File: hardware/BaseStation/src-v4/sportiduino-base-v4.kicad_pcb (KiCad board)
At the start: 2 copper layers, 73 x 45 mm, 46 parts, among them SW1 SW_Reed, X1 Battery, X2 Prog, X3 RC522, X4 MINI RC522, X5 Charge

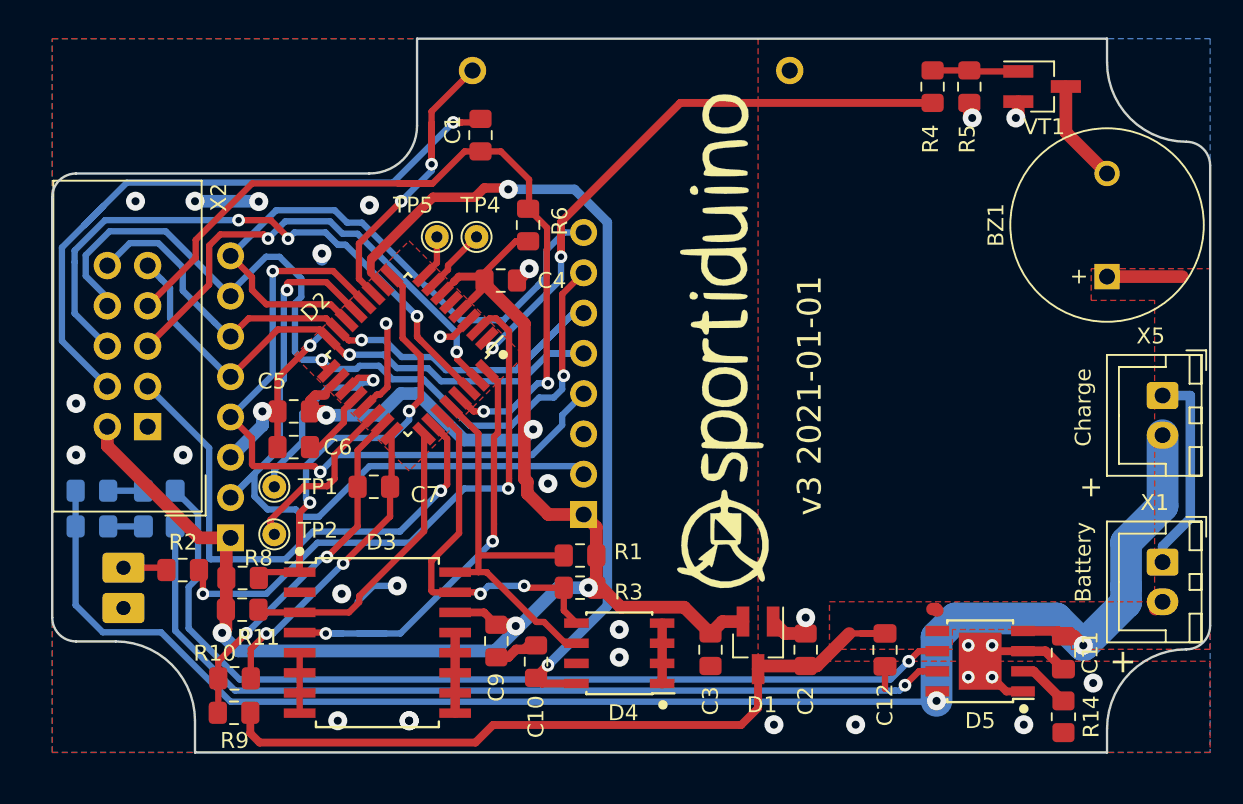
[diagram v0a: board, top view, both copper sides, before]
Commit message: New PCB (wip)
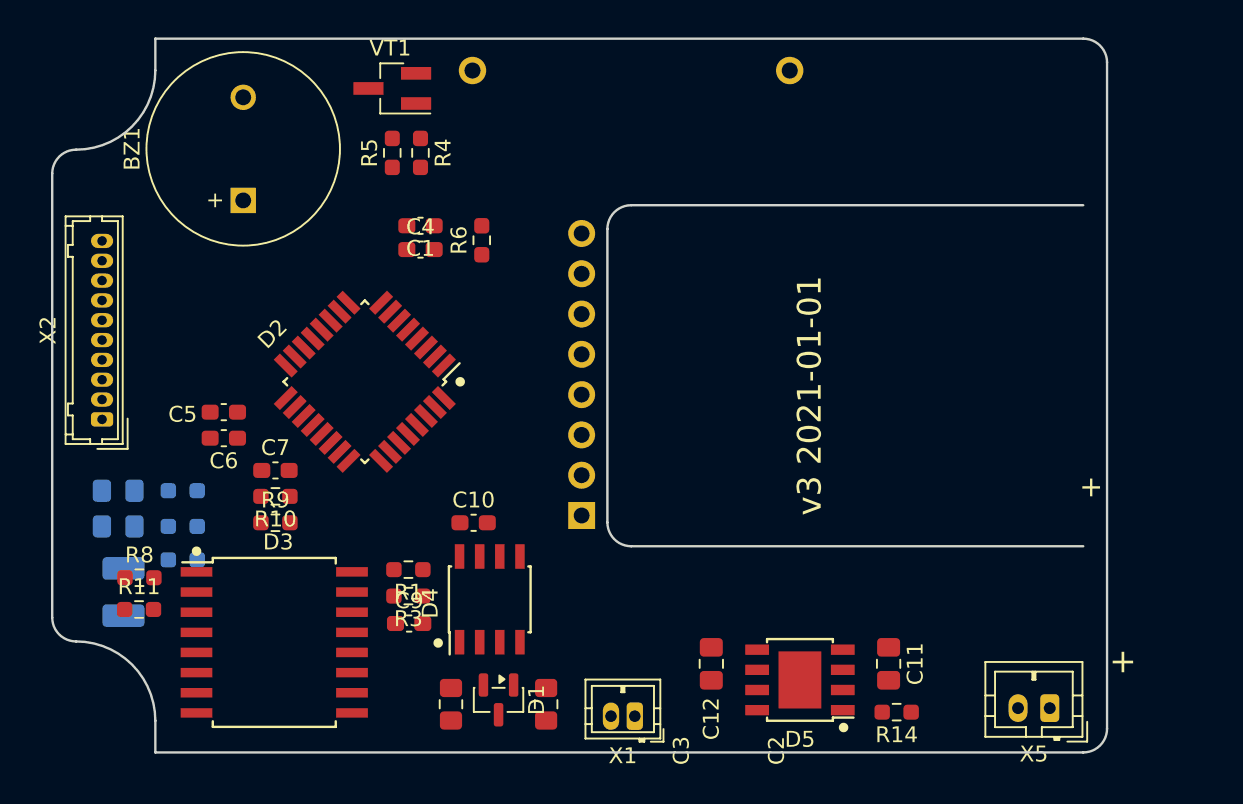
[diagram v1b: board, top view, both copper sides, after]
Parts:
- removed G*** (x2): LOGO, Sportiduino:logo
- removed TP1, TP2, TP4, TP5: , TestPoint:TestPoint_THTPad_D1.5mm_Drill0.7mm
- removed X4: MINI RC522, Connector_PinHeader_2.54mm:PinHeader_1x08_P2.54mm_Vertical
- C1, C10, C4, C5, C6, C7, C9: footprint Capacitor_SMD:C_0805_2012Metric_Pad1.15x1.40mm_HandSolder -> Capacitor_SMD:C_0603_1608Metric_Pad1.08x0.95mm_HandSolder
- D1: footprint Package_TO_SOT_SMD:SOT-23_Handsoldering -> Package_TO_SOT_SMD:SOT-23
- R1, R10, R11, R3, R4, R5, R6, R8, R9: footprint Resistor_SMD:R_0805_2012Metric_Pad1.15x1.40mm_HandSolder -> Resistor_SMD:R_0603_1608Metric_Pad0.98x0.95mm_HandSolder
- R12, R13, R14: footprint Resistor_SMD:R_0805_2012Metric_Pad1.20x1.40mm_HandSolder -> Resistor_SMD:R_0603_1608Metric_Pad0.98x0.95mm_HandSolder
- R2: footprint Resistor_SMD:R_0805_2012Metric_Pad1.15x1.40mm_HandSolder -> Resistor_SMD:R_0603_1608Metric_Pad0.98x0.95mm_HandSolder; moved to B.Cu
- VD1: footprint LED_THT:LED_D3.0mm -> LED_SMD:LED_1210_3225Metric_Pad1.42x2.65mm_HandSolder
- VD2, VD3: value (none) -> 0805
- X1: footprint Connector_JST:JST_XH_B2B-XH-A_1x02_P2.50mm_Vertical -> Connector_JST:JST_ZH_B2B-ZR_1x02_P1.50mm_Vertical
- X2: footprint Connector_IDC:IDC-Header_2x05_P2.54mm_Vertical -> Connector_Hirose:Hirose_DF13-10P-1.25DSA_1x10_P1.25mm_Vertical
- X3: value RC522 -> MINI RC522
- X5: footprint Connector_JST:JST_XH_B2B-XH-A_1x02_P2.50mm_Vertical -> Connector_JST:JST_PH_B2B-PH-K_1x02_P2.00mm_Vertical
- moved BZ1 54.7 mm to (145.6, 68.6)
- moved VT1 41.0 mm to (155.0, 61.6), turned to 180 degrees
- moved R5 36.6 mm to (155.0, 65.6)
- moved X1 34.7 mm to (170.3, 101.2), turned to 180 degrees
- moved R4 32.6 mm to (156.8, 65.6)
- moved X3 22.2 mm to (166.9, 88.5)
- moved X5 21.0 mm to (196.4, 100.6), turned to 180 degrees
- moved D1 16.7 mm to (161.7, 100.1)
- moved C2 16.7 mm to (164.7, 100.4)
- moved C3 16.7 mm to (158.7, 100.4)
- moved R9 12.3 mm to (147.6, 89.0)
- moved R10 11.8 mm to (147.6, 87.3)
- moved D5 11.4 mm to (180.7, 98.9)
- moved C11 11.0 mm to (186.3, 97.9)
- moved C12 11.0 mm to (175.1, 97.9)
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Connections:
- C1 pad 2: Net-(C1-Pad2) -> Net-(X2-Pin_10)
- D2 pad 19: Net-(D2-Pad19) -> unconnected-(D2-ADC6-Pad19)
- D2 pad 22: Net-(D2-Pad22) -> unconnected-(D2-ADC7-Pad22)
- D2 pad 7: Net-(D2-Pad7) -> unconnected-(D2-XTAL1/PB6-Pad7)
- D2 pad 8: Net-(D2-Pad8) -> unconnected-(D2-XTAL2/PB7-Pad8)
- X2 pad 10: PB3 -> Net-(X2-Pin_10)
- X2 pad 3: PC3 -> RST
- X2 pad 4: Net-(C1-Pad2) -> PB5
- X2 pad 5: TX -> PB3
- X2 pad 6: RX -> PB4
- X2 pad 7: RST -> PC3
- X2 pad 8: PB5 -> TX
- X2 pad 9: PB4 -> RX
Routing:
- net +3V3: track 114.9 -> 0.00 mm, vias 5 -> 0
- net Net-(D5-CE): track 98.0 -> 0.00 mm, vias 2 -> 0
- net GNDD: track 72.1 -> 0.00 mm, vias 32 -> 0
- net Net-(D5-~{STDBY}): track 58.8 -> 0.00 mm, vias 1 -> 0
- net Net-(D5-~{CHRG}): track 56.7 -> 0.00 mm, vias 1 -> 0
- net PB5: track 56.4 -> 0.00 mm, vias 2 -> 0
- net +BATT: track 54.0 -> 0.00 mm
- net PD6: track 52.8 -> 0.00 mm, vias 2 -> 0
- net RST: track 52.7 -> 0.00 mm, vias 2 -> 0
- net /PB1: track 49.1 -> 0.00 mm, vias 1 -> 0
- net /PB0: track 45.3 -> 0.00 mm, vias 2 -> 0
- net PB3: track 43.1 -> 0.00 mm, vias 1 -> 0
- net /PB2: track 42.2 -> 0.00 mm
- net Net-(C1-Pad2): track 41.1 -> 0.00 mm, vias 1 -> 0
- net RX: track 39.3 -> 0.00 mm, vias 3 -> 0
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- removed copper zone on F.Cu, net +BATT
- removed copper zone on B.Cu, net GNDD
- removed copper zone on F.Cu, net GNDD
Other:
- board size 73 x 45 mm -> 66.5 x 45 mm
- net class Default removed
- net class power removed
- board text removed: "Ali 83x58mm"
- board text removed: "RC522"

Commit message: pcb wip
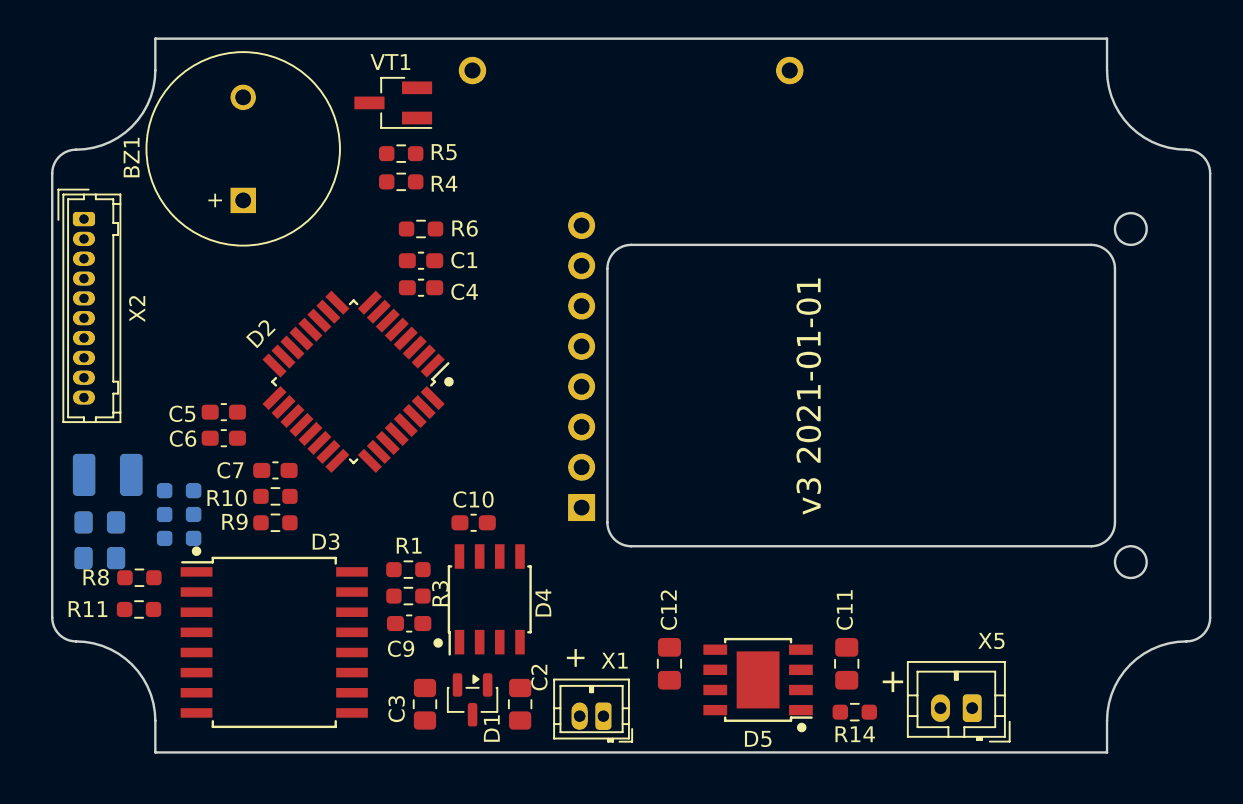
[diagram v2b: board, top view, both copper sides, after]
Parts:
- moved X2 12.7 mm to (135.5, 69.8), turned to -90 degrees
- moved VD1 7.45 mm to (137.0, 85.9), turned to 0 degrees
- moved X5 4.89 mm to (191.5, 100.6)
- moved R2 4.36 mm to (141.5, 86.9), turned to 0 degrees
- moved R6 3.89 mm to (156.8, 70.4), turned to 0 degrees
- moved C12 2.64 mm to (172.4, 97.9)
- moved D5 2.64 mm to (178.0, 98.9)
- moved R14 2.64 mm to (184.1, 100.9)
- moved C11 2.64 mm to (183.6, 97.9)
- moved C4 2.40 mm to (156.8, 74.1)
- moved VD2 2.31 mm to (136.5, 88.9)
- moved VD3 2.31 mm to (136.5, 91.2)
- moved C1 2.20 mm to (156.8, 72.4)
- moved R4 2.19 mm to (155.5, 67.5), turned to 180 degrees
- moved X1 1.98 mm to (168.3, 101.2)
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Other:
- board size 66.5 x 45 mm -> 73 x 45 mm
